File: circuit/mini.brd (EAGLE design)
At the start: 100 x 80 mm, 79 parts, among them IC1 74AC4053D, IC2 74AC74D, IC3 STM32L151CBT6, IC4 MCP1700-3.3V, IC5 NE5534D, IC6 NE5534D, Q1 BFG135, Q2 8MHz, X1 1-227161-0, X4 MINI-USB

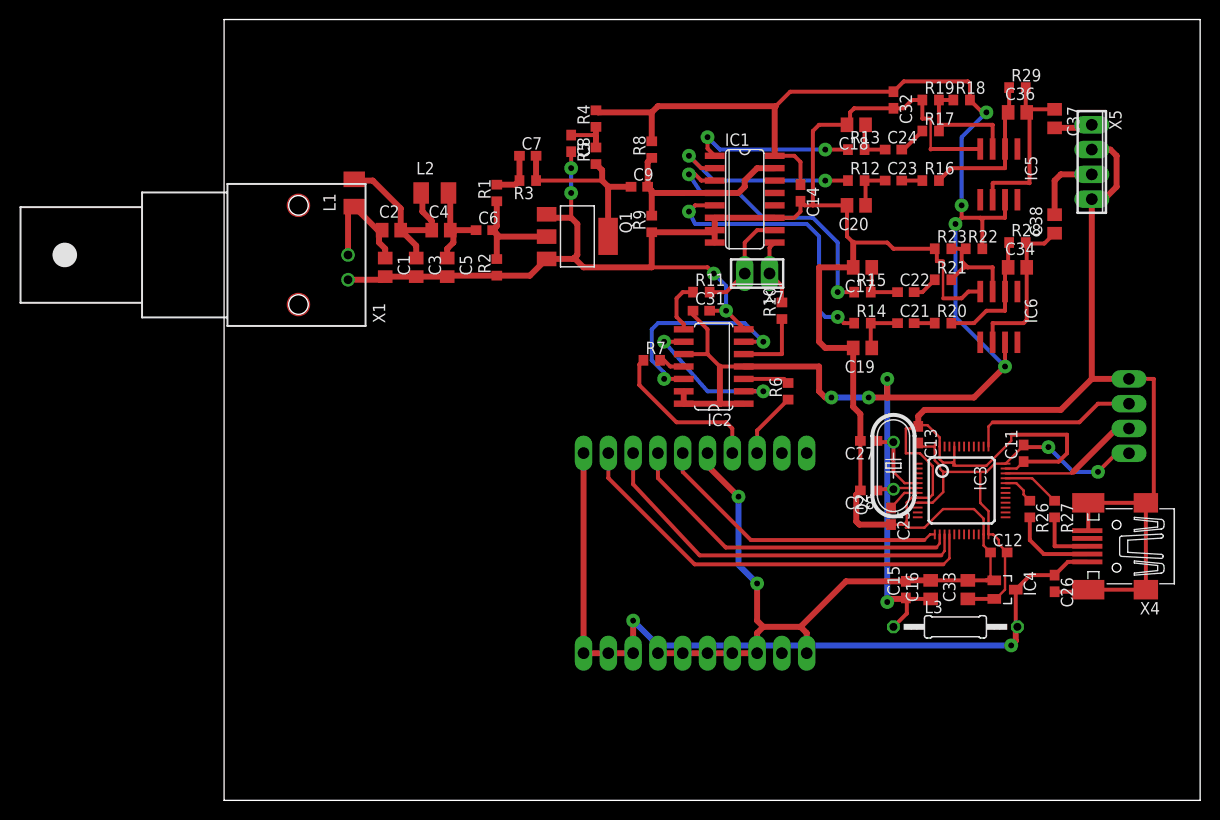
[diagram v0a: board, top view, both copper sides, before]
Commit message: - ?????????????????? ?? ??????? 85x60??
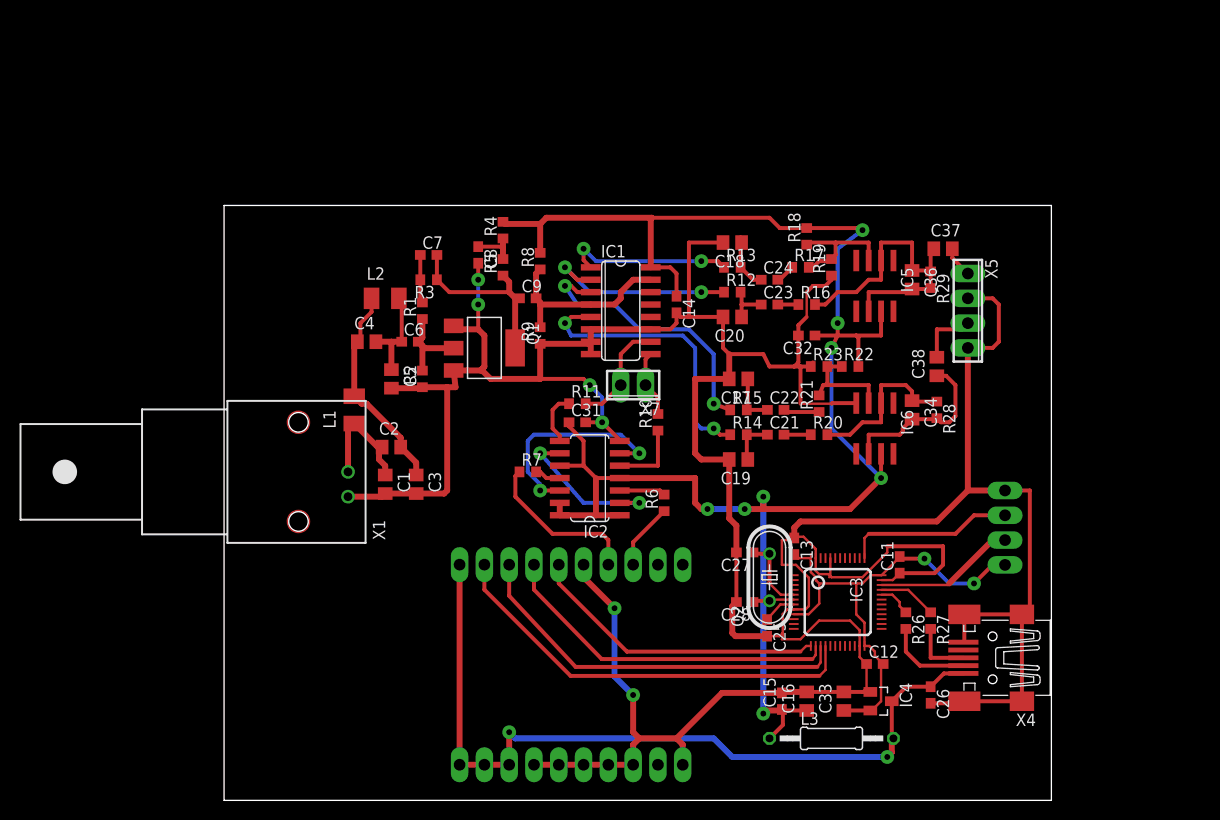
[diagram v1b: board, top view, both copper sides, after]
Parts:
- moved C32 25.7 mm to (59.7, 47.6), turned to 180 degrees
- moved C1 22.2 mm to (16.5, 32.4)
- moved C2 22.2 mm to (17.1, 36.2)
- moved C3 22.2 mm to (19.7, 32.4)
- moved X1 22.2 mm to (7.62, 33.7)
- moved L1 22.2 mm to (13.3, 40.0)
- moved R29 21.6 mm to (72.4, 53.3), turned to 270 degrees
- moved R18 21.1 mm to (59.7, 57.8), turned to 90 degrees
- moved C36 20.3 mm to (70.5, 53.3), turned to 270 degrees
- moved R19 19.9 mm to (62.2, 54.6), turned to 90 degrees
- moved X5 19.8 mm to (76.2, 50.2)
- moved R17 19.3 mm to (59.1, 54.6)
- moved R28 19.0 mm to (73.0, 40.0), turned to 270 degrees
- moved C38 18.9 mm to (73.0, 44.5)
- moved C24 18.4 mm to (55.9, 53.3)
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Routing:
- net GND: track 404.8 -> 397.9 mm
- net N$18: track 18.4 -> 12.6 mm
- net +5V: track 185.3 -> 180.4 mm
- net N$17: track 15.7 -> 19.6 mm
- net N$22: track 13.2 -> 16.8 mm
- net N$41: track 19.2 -> 21.9 mm
- net N$44: track 12.1 -> 9.53 mm
- net N$13: track 4.69 -> 6.26 mm
- net N$39: track 7.57 -> 6.30 mm
- net N$6: track 20.3 -> 19.0 mm
- net N$21: track 2.64 -> 3.68 mm
- net N$25: track 2.90 -> 2.00 mm
- net N$16: track 16.9 -> 17.7 mm
- net N$34: track 19.6 -> 18.8 mm
- net N$38: track 3.94 -> 3.20 mm
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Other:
- board size 100 x 80 mm -> 84.8 x 61 mm
